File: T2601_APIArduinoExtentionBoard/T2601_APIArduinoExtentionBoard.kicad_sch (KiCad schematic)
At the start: 95 parts, among them J1 Conn_01x10_Socket, J11 Conn_01x04_Pin, J12 Screw_Terminal_01x02, J13 Conn_01x04_Pin, J14 Screw_Terminal_01x02, J15 Conn_02x08_Counter_Clockwise, J2 Conn_01x10_Socket, J3 Conn_01x10_Socket, J4 Conn_01x10_Socket, J5 Screw_Terminal_01x08, J6 Screw_Terminal_01x08, J7 Conn_02x03_Counter_Clockwise, J8 Conn_01x04, J9 Conn_02x08_Counter_Clockwise, U1 ATMEGA328P-AU, U2 ATmega328PB-A, X1 X322516MOB4SI

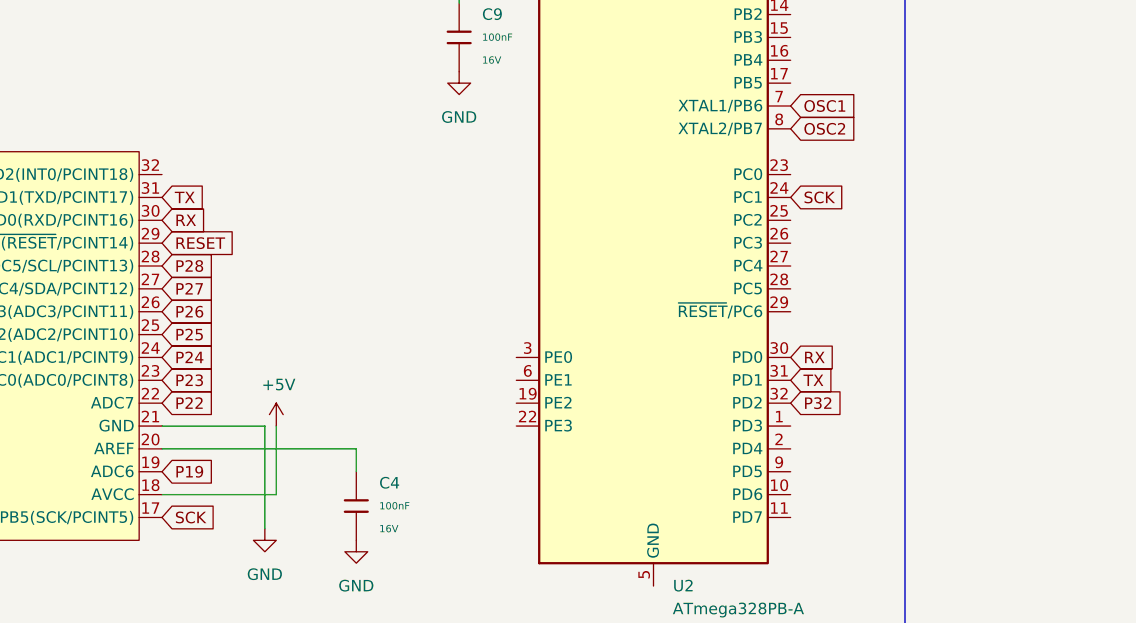
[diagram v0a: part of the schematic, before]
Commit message: kicad modif
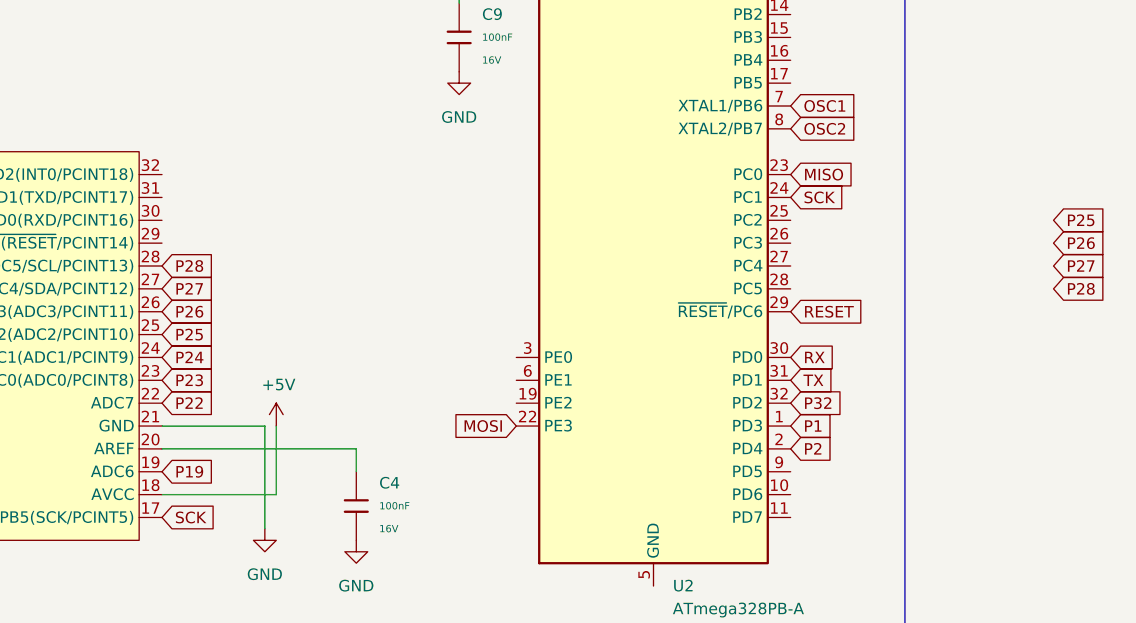
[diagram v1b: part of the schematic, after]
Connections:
- net MISO: now also U2.23 (PC0)
- net MOSI: now also U2.22 (PE3)
- net P1: now also U2.1 (PD3)
- net P2: now also U2.2 (PD4)
- net RESET: now also U2.29 (~{RESET}/PC6); no longer U1.29 (~{PC6(RESET}/PCINT14))
- net RX: no longer U1.30 (PD0(RXD/PCINT16))
- net TX: no longer U1.31 (PD1(TXD/PCINT17))
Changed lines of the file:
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@@
+		)
+	)
+	(global_label "P25"
+		(shape input)
+		(at 365.76 294.64 0)
+		(fields_autoplaced yes)
+		(effects
+			(font
+				(size 1.27 1.27)
+			)
+			(justify left)
+		)
+		(property "Intersheetrefs" "${INTERSHEET_REFS}"
+			(at 372.4342 294.64 0)
+			(hide yes)
+			(show_name no)
+			(do_not_autoplace no)
+			(effects
+				(font
+					(size 1.27 1.27)
+				)
+				(justify left)
+			)
 		)
 	)
@@
 		)
 	)
+	(global_label "MOSI"
+		(shape input)
+		(at 306.07 317.5 180)
+		(fields_autoplaced yes)
+		(effects
+			(font
+				(size 1.27 1.27)
+			)
+			(justify right)
+		)
+		(property "Intersheetrefs" "${INTERSHEET_REFS}"
+			(at 298.4886 317.5 0)
+			(hide yes)
+			(show_name no)
+			(do_not_autoplace no)
+			(effects
+				(font
+					(size 1.27 1.27)
+				)
+				(justify right)
+			)
+		)
+	)
 	(global_label "P12"
 		(shape input)
@@
 		)
 	)
+	(global_label "P27"
+		(shape input)
+		(at 365.76 299.72 0)
+		(fields_autoplaced yes)
+		(effects
+			(font
+				(size 1.27 1.27)
+			)
+			(justify left)
+		)
+		(property "Intersheetrefs" "${INTERSHEET_REFS}"
+			(at 372.4342 299.72 0)
+			(hide yes)
+			(show_name no)
+			(do_not_autoplace no)
+			(effects
+				(font
+					(size 1.27 1.27)
+				)
+				(justify left)
+			)
+		)
+	)
 	(global_label "TX_DEBUG"
 		(shape input)
@@
 	(global_label "RESET"
 		(shape input)
-		(at 266.7 297.18 0)
-		(fields_autoplaced yes)
-		(effects
-			(font
-				(size 1.27 1.27)
-			)
-			(justify left)
-		)
-		(property "Intersheetrefs" "${INTERSHEET_REFS}"
-			(at 275.4303 297.18 0)
+		(at 336.55 304.8 0)
+		(fields_autoplaced yes)
+		(effects
+			(font
+				(size 1.27 1.27)
+			)
+			(justify left)
+		)
+		(property "Intersheetrefs" "${INTERSHEET_REFS}"
+			(at 345.2803 304.8 0)
 			(hide yes)
 			(show_name no)
@@
 		)
 	)
+	(global_label "MISO"
+		(shape input)
+		(at 336.55 289.56 0)
+		(fields_autoplaced yes)
+		(effects
+			(font
+				(size 1.27 1.27)
+			)
+			(justify left)
+		)
+		(property "Intersheetrefs" "${INTERSHEET_REFS}"
+			(at 344.1314 289.56 0)
+			(hide yes)
+			(show_name no)
+			(do_not_autoplace no)
+			(effects
+				(font
+					(size 1.27 1.27)
+				)
+				(justify left)
+			)
+		)
+	)
 	(global_label "P1"
 		(shape input)
@@
 		)
 	)
+	(global_label "P1"
+		(shape input)
+		(at 336.55 317.5 0)
+		(fields_autoplaced yes)
+		(effects
+			(font
+				(size 1.27 1.27)
+			)
+			(justify left)
+		)
+		(property "Intersheetrefs" "${INTERSHEET_REFS}"
+			(at 342.0147 317.5 0)
+			(hide yes)
+			(show_name no)
+			(do_not_autoplace no)
+			(effects
+				(font
+					(size 1.27 1.27)
+				)
+				(justify left)
+			)
+		)
+	)
 	(global_label "P13"
 		(shape input)
@@
 		)
 	)
+	(global_label "P2"
+		(shape input)
+		(at 336.55 320.04 0)
+		(fields_autoplaced yes)
+		(effects
+			(font
+				(size 1.27 1.27)
+			)
+			(justify left)
+		)
+		(property "Intersheetrefs" "${INTERSHEET_REFS}"
+			(at 342.0147 320.04 0)
+			(hide yes)
+			(show_name no)
+			(do_not_autoplace no)
+			(effects
+				(font
+					(size 1.27 1.27)
+				)
+				(justify left)
+			)
+		)
+	)
+	(global_label "P28"
+		(shape input)
+		(at 365.76 302.26 0)
+		(fields_autoplaced yes)
+		(effects
+			(font
+				(size 1.27 1.27)
+			)
+			(justify left)
+		)
+		(property "Intersheetrefs" "${INTERSHEET_REFS}"
+			(at 372.4342 302.26 0)
+			(hide yes)
+			(show_name no)
+			(do_not_autoplace no)
+			(effects
+				(font
+					(size 1.27 1.27)
+				)
+				(justify left)
+			)
+		)
+	)
 	(global_label "P14"
 		(shape input)
@@
 		)
 	)
-	(global_label "TX"
-		(shape input)
-		(at 266.7 292.1 0)
-		(fields_autoplaced yes)
-		(effects
-			(font
-				(size 1.27 1.27)
-			)
-			(justify left)
-		)
-		(property "Intersheetrefs" "${INTERSHEET_REFS}"
-			(at 271.8623 292.1 0)
-			(hide yes)
-			(show_name no)
-			(do_not_autoplace no)
-			(effects
-				(font
-					(size 1.27 1.27)
-				)
-				(justify left)
-			)
-		)
-	)
 	(global_label "P11"
 		(shape input)
@@
 		)
 	)
+	(global_label "P26"
+		(shape input)
+		(at 365.76 297.18 0)
+		(fields_autoplaced yes)
+		(effects
+			(font
+				(size 1.27 1.27)
+			)
+			(justify left)
+		)
+		(property "Intersheetrefs" "${INTERSHEET_REFS}"
+			(at 372.4342 297.18 0)
+			(hide yes)
+			(show_name no)
+			(do_not_autoplace no)
+			(effects
+				(font
+					(size 1.27 1.27)
+				)
+				(justify left)
+			)
+		)
+	)
 	(global_label "MISO"
 		(shape input)
@@
 			(hide yes)
 			(show_name no)
-			(do_not_autoplace no)
-			(effects
-				(font
-					(size 1.27 1.27)
-				)
-				(justify left)
-			)
-		)
-	)
-	(global_label "RX"
-		(shape input)
-		(at 266.7 294.64 0)
-		(fields_autoplaced yes)
-		(effects
-			(font
-				(size 1.27 1.27)
-			)
-			(justify left)
-		)
-		(property "Intersheetrefs" "${INTERSHEET_REFS}"
-			(at 272.1647 294.64 0)
-			(hide yes)
-			(show_name no)
